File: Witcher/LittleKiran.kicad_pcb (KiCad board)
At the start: 2 copper layers, 34.7 x 34.7 mm, 11 parts, among them J1 XT60PW-M, J2 XT60PW-M, J3 XT60PW-M, Q1 PXP012-30QLJ, Q2 PXP012-30QLJ, U1 LTC4412xS6, U2 LTC4412xS6

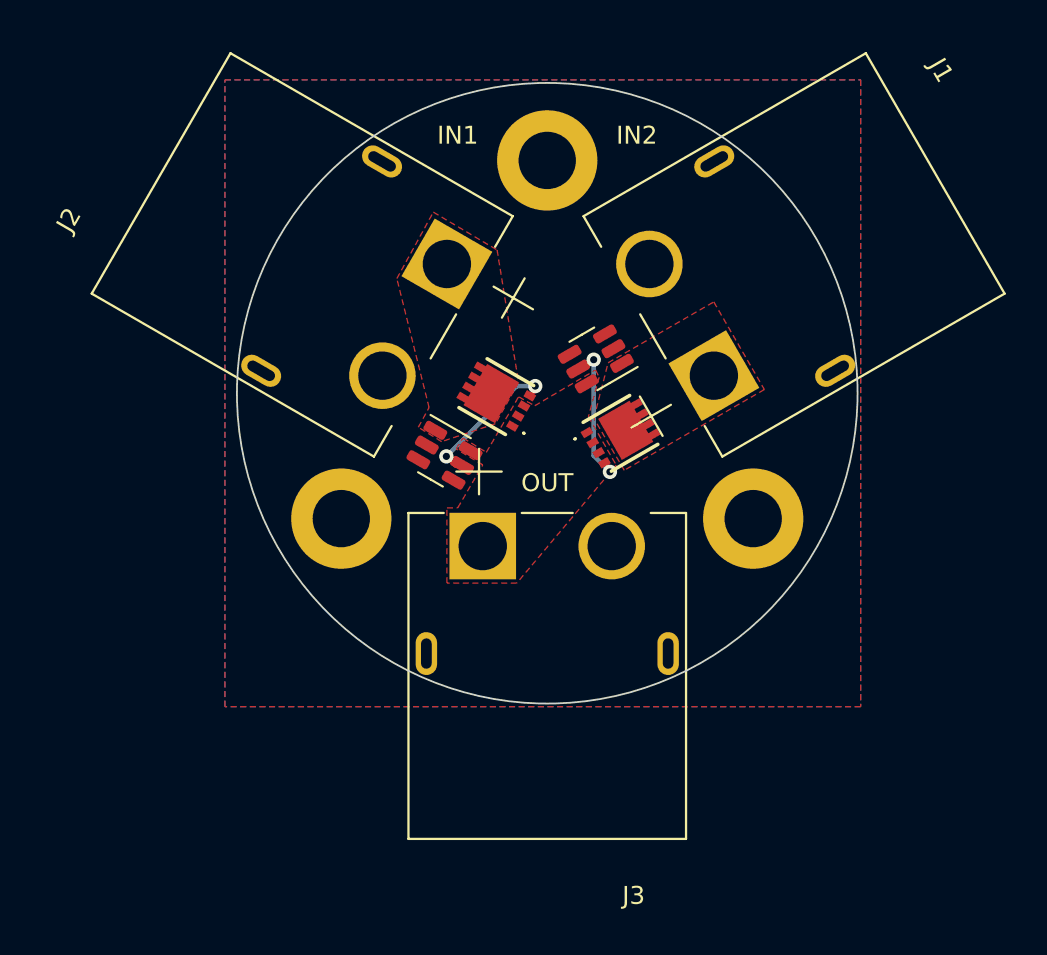
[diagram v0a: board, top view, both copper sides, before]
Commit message: finito
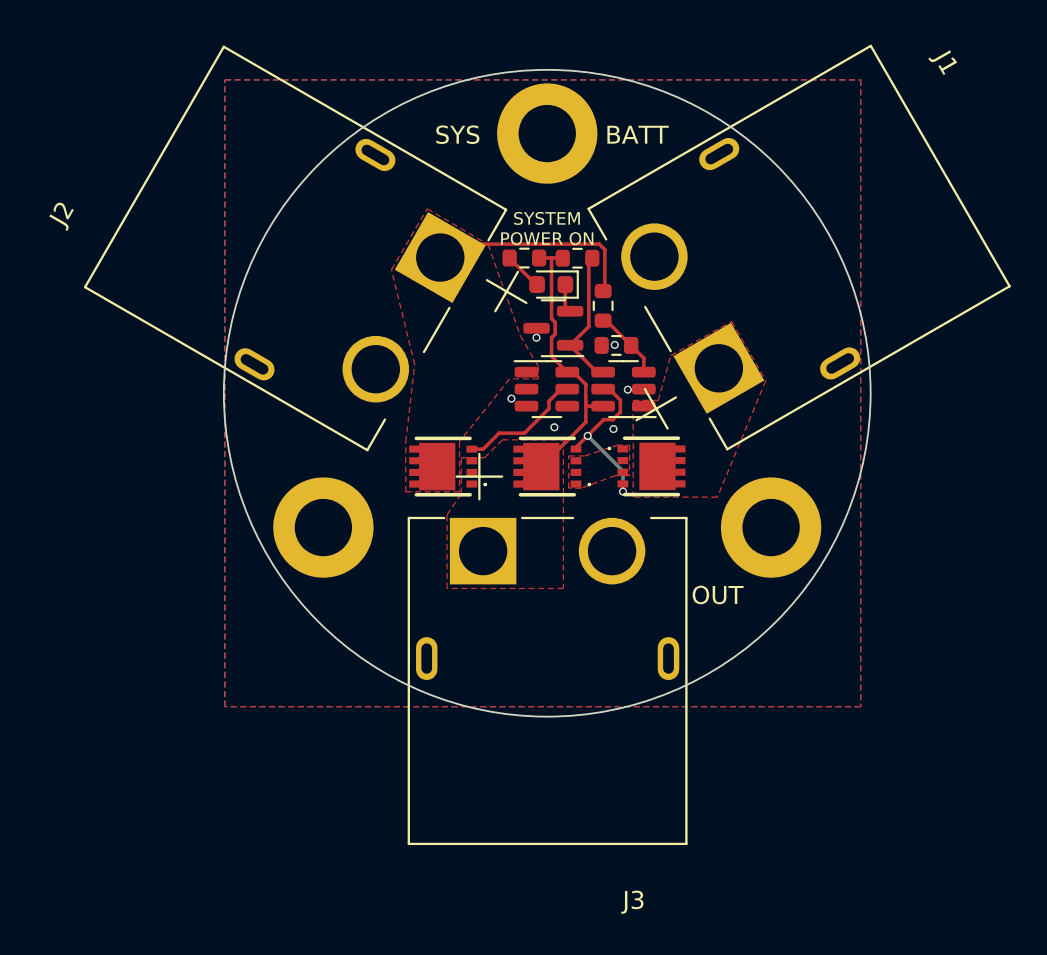
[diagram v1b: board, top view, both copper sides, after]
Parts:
- added D1: SYS_LED, LED_SMD:LED_0603_1608Metric, F.Cu at (129.7, 75.4)
- added Q3: PXP012-30QLJ, iclr:PXP01230QLJ, F.Cu at (129.5, 85.6)
- added Q4: FDN340P, Package_TO_SOT_SMD:SOT-23, F.Cu at (129.8, 77.9)
- added R1: 0, Resistor_SMD:R_0603_1608Metric, F.Cu at (132.6, 76.6)
- added R2: 10k, Resistor_SMD:R_0603_1608Metric, F.Cu at (133.4, 78.8)
- added R3: 470k, Resistor_SMD:R_0603_1608Metric, F.Cu at (131.2, 74.0)
- added R4: 3k, Resistor_SMD:R_0603_1608Metric, F.Cu at (128.2, 74.0)
- moved U2 6.81 mm to (129.5, 81.3), turned to 0 degrees
- moved Q1 4.90 mm to (123.7, 85.6), turned to 90 degrees
- moved Q2 2.53 mm to (135.3, 85.6), turned to -90 degrees
- moved U1 2.29 mm to (133.8, 81.3), turned to 180 degrees
- moved H2 1.50 mm to (129.5, 67.0)
- moved H1 1.12 mm to (142.0, 89.0)
- moved H3 1.12 mm to (117.0, 89.0)
- moved J2 0.52 mm to (116.5, 74.0)
- moved J1 0.50 mm to (142.5, 74.0)
- moved J3 0.28 mm to (129.5, 96.3)
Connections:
- net Net-(Q2-G) renamed /GATE1
- J3 pad 1: Net-(J3-+) -> /SENSE
- Q1 pad 1: Net-(J3-+) -> /SENSE
- Q1 pad 2: Net-(J3-+) -> /SENSE
- Q1 pad 3: Net-(J3-+) -> /SENSE
- Q2 pad 1: Net-(J3-+) -> Net-(Q2-S_1)
- Q2 pad 2: Net-(J3-+) -> Net-(Q2-S_1)
- Q2 pad 3: Net-(J3-+) -> Net-(Q2-S_1)
- U1 pad 3: GND -> Net-(U1-CTL)
- U1 pad 4: unconnected-(U1-STAT-Pad4) -> /STAT
- U1 pad 6: Net-(J3-+) -> /SENSE
- U2 pad 6: Net-(J3-+) -> /SENSE
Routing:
- net /SENSE: track 0.00 -> 16.1 mm
- net Net-(J2-+): track 0.00 -> 12.0 mm
- net /STAT: track 0.00 -> 7.84 mm
- net Net-(U1-CTL): track 0.00 -> 3.92 mm
- net Net-(D1-A): track 0.00 -> 2.15 mm
- net Net-(D1-K): track 0.00 -> 1.60 mm
- net Net-(Q1-G): track 8.35 -> 6.96 mm, vias 2 -> 0
- net /GATE1: track 8.36 -> 9.64 mm
- net GND: vias 0 -> 6
- added copper zone on F.Cu, net /SENSE
- added copper zone on F.Cu, net Net-(Q2-S_1)
- removed copper zone on F.Cu, net Net-(J3-+)
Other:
- board size 34.7 x 34.7 mm -> 36.1 x 36.1 mm
- board text added: "BATT"
- board text added: "SYS"
- board text added: "SYSTEM POWER ON"
- board text removed: "IN1"
- board text removed: "IN2"
